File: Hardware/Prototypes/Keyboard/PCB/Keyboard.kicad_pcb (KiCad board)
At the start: 2 copper layers, 32 x 18 mm, 25 parts, among them P1 USB_OTG, SW1 RESET, U1 ATMEGA32U4-QFN44, X1 ABM10-16.000MHZ-D30-T3

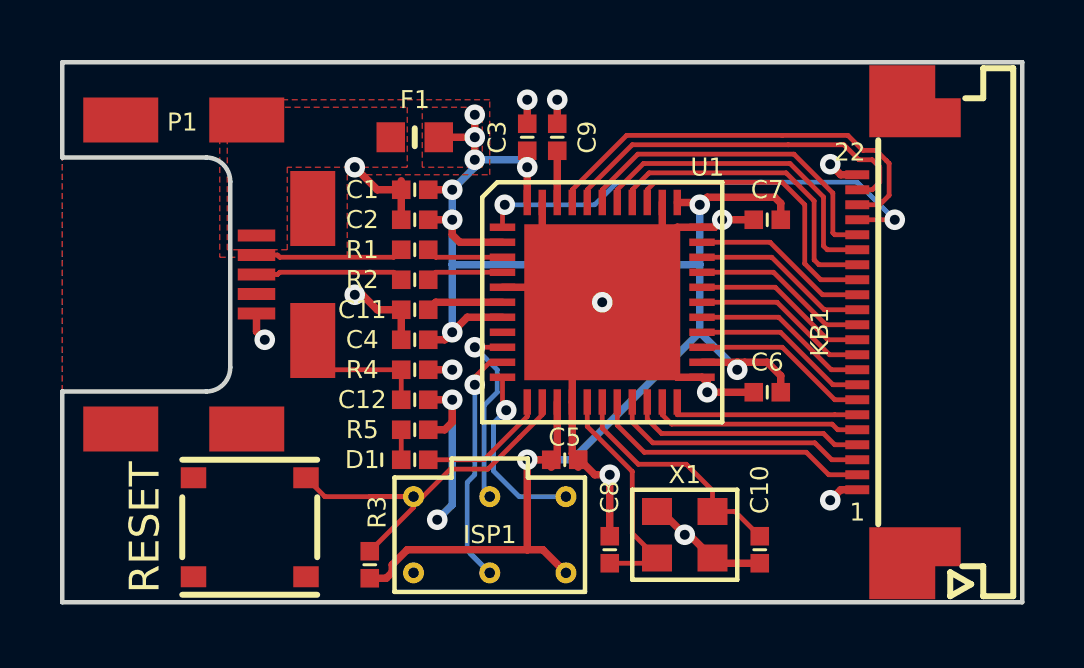
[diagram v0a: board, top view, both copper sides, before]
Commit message: Major data dump
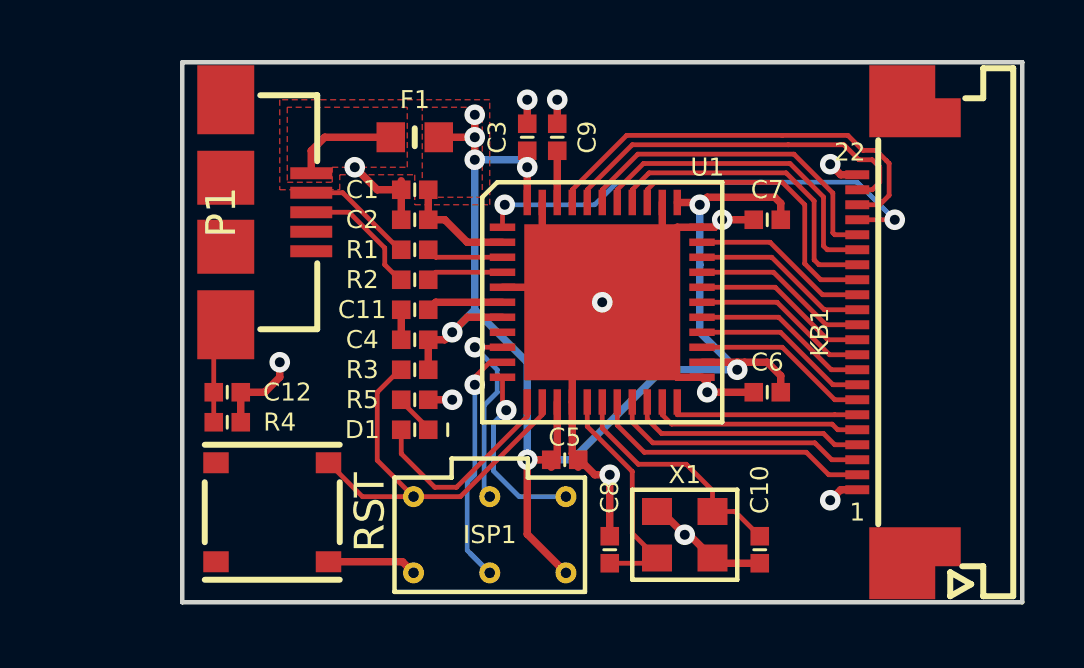
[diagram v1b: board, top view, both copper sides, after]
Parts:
- P1: footprint SMD-Connectors:USB-MICRO-MOLEX-47491-0001 -> SMD-Connectors:USB-MICRO-10104110-0001LF
- SW1: value RESET -> RST
- moved R3 6.67 mm to (156.8, 108.2), turned to 180 degrees
- moved R4 6.49 mm to (150.5, 110.0)
- moved C12 6.25 mm to (150.5, 109.0)
- moved P1 4.51 mm to (149.0, 103.0)
- moved D1 1.00 mm to (156.8, 110.2), turned to 180 degrees
- moved R5 1.00 mm to (156.8, 109.2)
- moved SW1 0.90 mm to (152.0, 113.0)
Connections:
- net Net-(P1-Pad2) renamed /BUS-
- net Net-(P1-Pad3) renamed /BUS+
- net Net-(R1-Pad2) renamed /D-
- net Net-(R2-Pad1) renamed /D+
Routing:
- net +5V: track 62.2 -> 55.2 mm, vias 10 -> 8
- net VBUS: track 0.00 -> 3.59 mm
- net GND: track 56.5 -> 53.1 mm, vias 15 -> 12
- net /LED: track 4.38 -> 7.35 mm
- net GNDPWR: track 5.58 -> 3.42 mm
- net /BUS-: track 5.21 -> 4.03 mm
- net /BUS+: track 5.21 -> 4.51 mm
- net /RESET: track 13.6 -> 14.2 mm
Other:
- board size 32 x 18 mm -> 28 x 18 mm
- rule pad_to_mask_clearance: 0.0762 -> 0.05
- rule solder_mask_min_width: 0.0762 -> 0.05
- board text added: "USB Keyboard v1.1 RasmusB 2017 Psion Series 5/5mx"
- board text removed: "USB Keyboard v1.1 RasmusB 2016 Psion Series 5/5mx"
